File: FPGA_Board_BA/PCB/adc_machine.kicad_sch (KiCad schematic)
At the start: 6 parts, among them J201 PinHeader_03_male, U201 LTC2320-16_LVDS

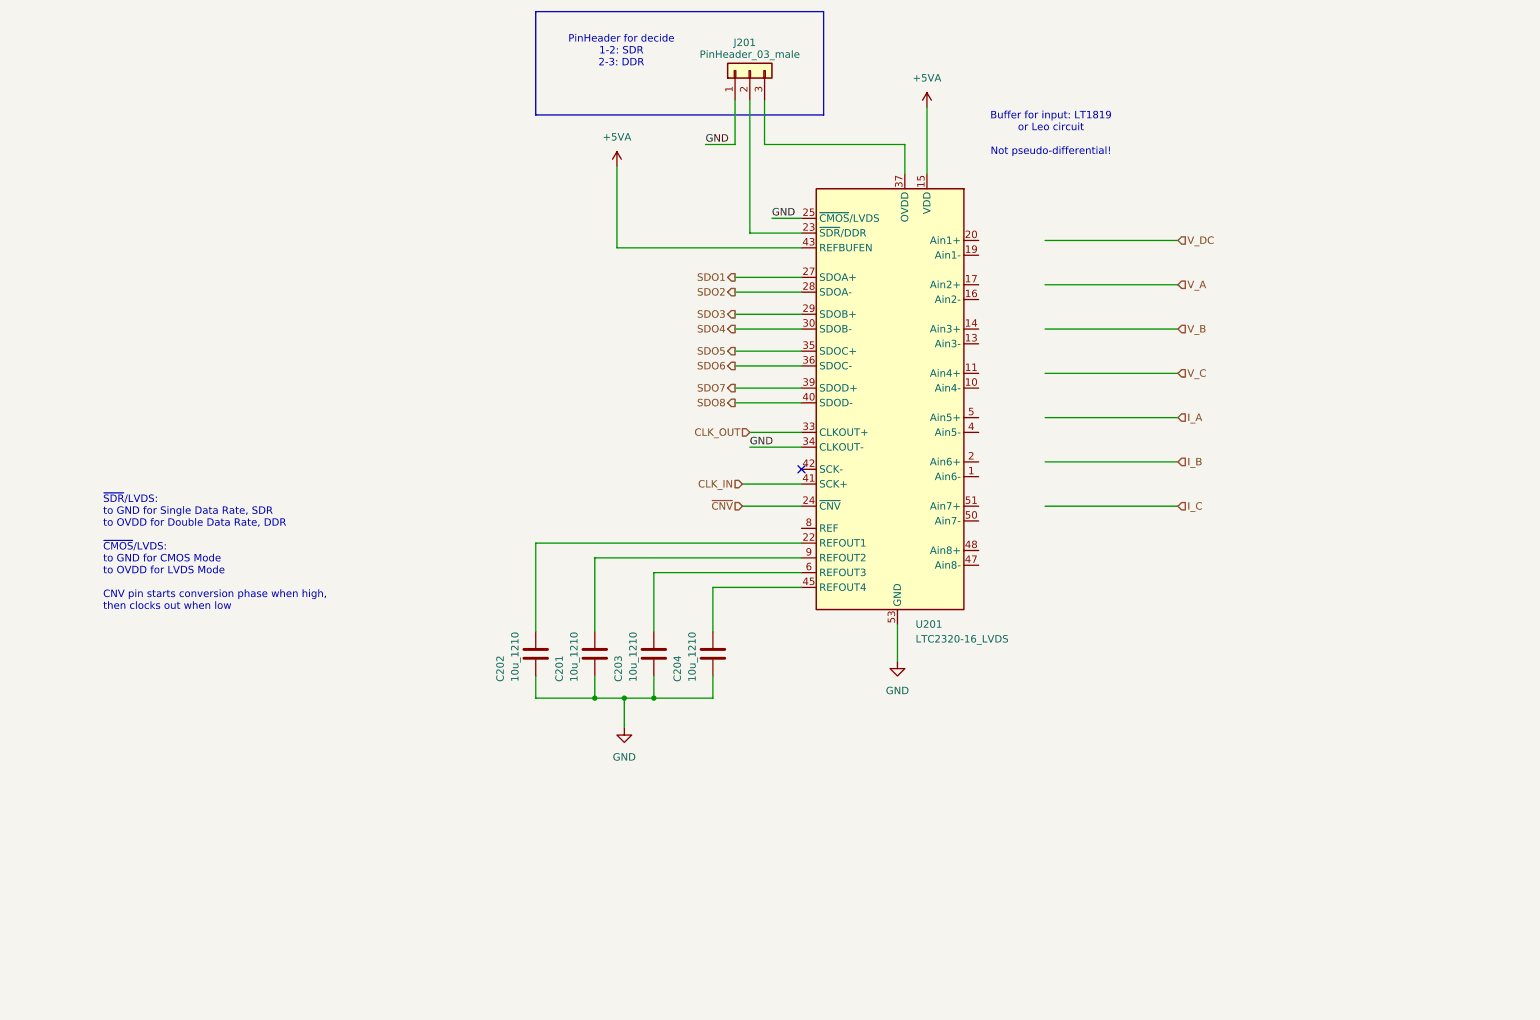
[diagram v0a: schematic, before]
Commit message: some schematic changes + Misc
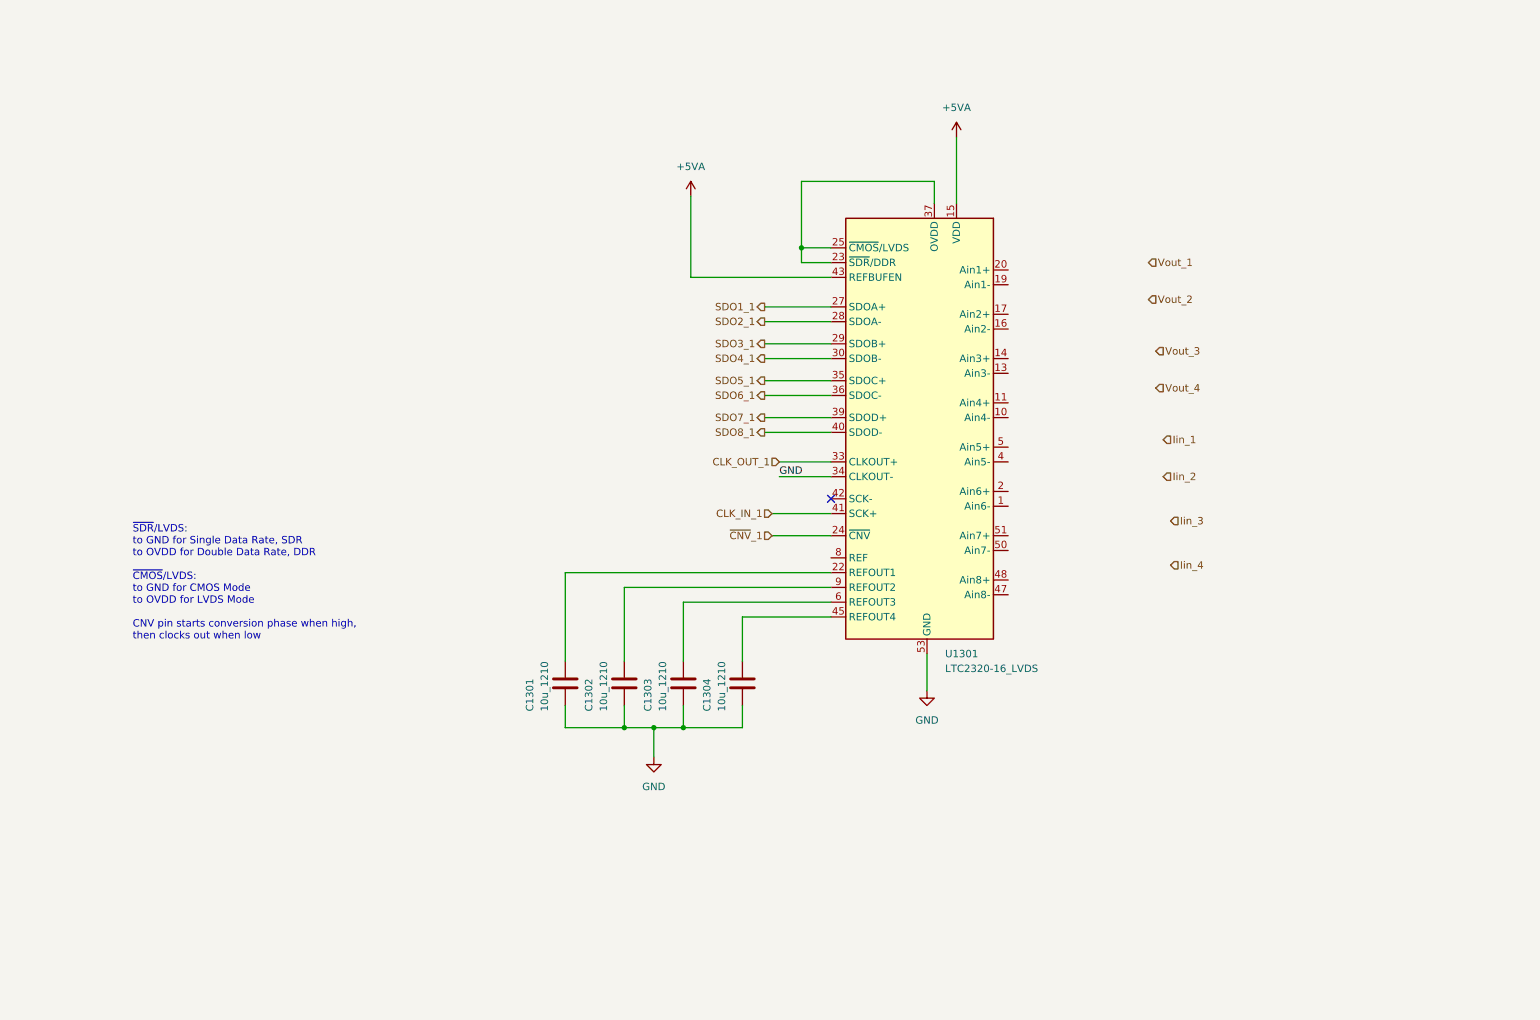
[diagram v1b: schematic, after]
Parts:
- removed C201, C202, C203, C204: 10u_1210, WLIB_Capacitor:C_1210, symbol WLIB_C:10u_1210
- removed J201: PinHeader_03_male, Connector_PinHeader_2.54mm:PinHeader_1x03_P2.54mm_Vertical, symbol WLIB_J:PinHeader_03_male
- removed U201: LTC2320-16_LVDS, MYLIB_chips:UKG_52_7mm_8mm, symbol MYLIB_U:LTC2320-16_LVDS
- added C1301, C1302, C1303, C1304: 10u_1210, WLIB_Capacitor:C_1210, symbol WLIB_C:10u_1210
- added U1301: LTC2320-16_LVDS, MYLIB_chips:UKG_52_7mm_8mm, symbol MYLIB_U:LTC2320-16_LVDS
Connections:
- net +5VA: now also U1301.15 (VDD), U1301.21 (VDD), U1301.43 (REFBUFEN), U1301.44 (VDD), U1301.52 (VDD)
- net GND: now also C1301.2, C1302.2, C1303.2, C1304.2, U1301.12 (GND), U1301.18 (GND), U1301.26 (GND), U1301.3 (GND), U1301.32 (GND), U1301.34 (CLKOUT-), U1301.38 (GND), U1301.46 (GND), U1301.49 (GND), U1301.53 (GND), U1301.7 (GND)
- net OVDD: now also U1301.23 (~{SDR}/DDR), U1301.25 (~{CMOS}/LVDS), U1301.31 (OVDD), U1301.37 (OVDD)
- new net: C1303.1, U1301.6 (REFOUT3)
- new net: C1301.1, U1301.22 (REFOUT1)
- new net: C1302.1, U1301.9 (REFOUT2)
- new net: C1304.1, U1301.45 (REFOUT4)
- new net CLK_IN_1: U1301.41 (SCK+)
- new net CLK_OUT_1: U1301.33 (CLKOUT+)
- new net SDO1_1: U1301.27 (SDOA+)
- new net SDO2_1: U1301.28 (SDOA-)
- new net SDO3_1: U1301.29 (SDOB+)
- new net SDO4_1: U1301.30 (SDOB-)
- new net SDO5_1: U1301.35 (SDOC+)
- new net SDO6_1: U1301.36 (SDOC-)
- new net SDO7_1: U1301.39 (SDOD+)
- new net SDO8_1: U1301.40 (SDOD-)
- new net ~{CNV}_1: U1301.24 (~{CNV})
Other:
- note removed: "Buffer for input: LT1819 or Leo circuit Not pseudo-differential!"
- note removed: "PinHeader for decide 1-2: SDR 2-3: DDR"

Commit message: lot of work
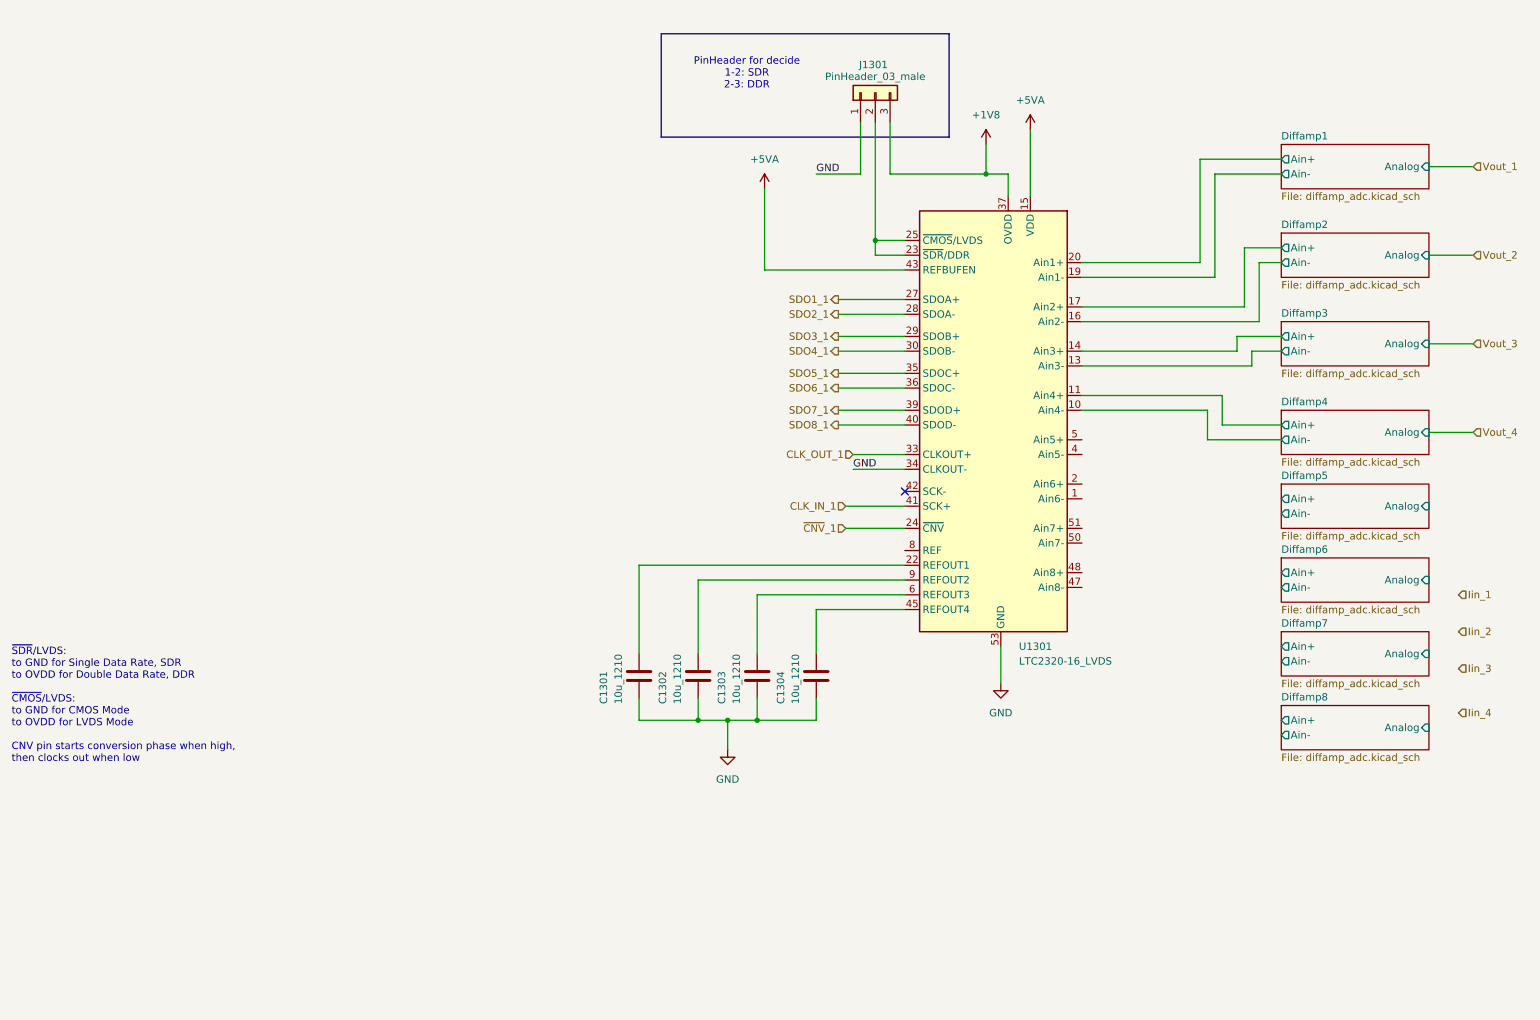
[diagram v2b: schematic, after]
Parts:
- added J1301: PinHeader_03_male, Connector_PinHeader_2.54mm:PinHeader_1x03_P2.54mm_Vertical, symbol WLIB_J:PinHeader_03_male
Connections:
- net GND: now also J1301.1 (Pin_1)
- net Diffamp4/Ain-: now reaches U1301.10 (Ain4-)
- net Diffamp4/Ain+: now reaches U1301.11 (Ain4+)
- net Diffamp3/Ain-: now reaches U1301.13 (Ain3-)
- net Diffamp3/Ain+: now reaches U1301.14 (Ain3+)
- net Diffamp2/Ain-: now reaches U1301.16 (Ain2-)
- net Diffamp2/Ain+: now reaches U1301.17 (Ain2+)
- net Diffamp1/Ain-: now reaches U1301.19 (Ain1-)
- net Diffamp1/Ain+: now reaches U1301.20 (Ain1+)
- net OVDD: no longer names the net of U1301.23 (~{SDR}/DDR), U1301.25 (~{CMOS}/LVDS)
- net OVDD: now also J1301.2 (Pin_2); no longer U1301.31 (OVDD), U1301.37 (OVDD)
- new net +1V8: J1301.3 (Pin_3), U1301.31 (OVDD), U1301.37 (OVDD)
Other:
- added sheet Diffamp1 (diffamp_adc.kicad_sch)
- added sheet Diffamp2 (diffamp_adc.kicad_sch)
- added sheet Diffamp3 (diffamp_adc.kicad_sch)
- added sheet Diffamp4 (diffamp_adc.kicad_sch)
- added sheet Diffamp5 (diffamp_adc.kicad_sch)
- added sheet Diffamp6 (diffamp_adc.kicad_sch)
- added sheet Diffamp7 (diffamp_adc.kicad_sch)
- added sheet Diffamp8 (diffamp_adc.kicad_sch)
- note added: "PinHeader for decide 1-2: SDR 2-3: DDR"
- moved on the sheet: C1301, C1302, C1303, C1304, U1301

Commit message: work
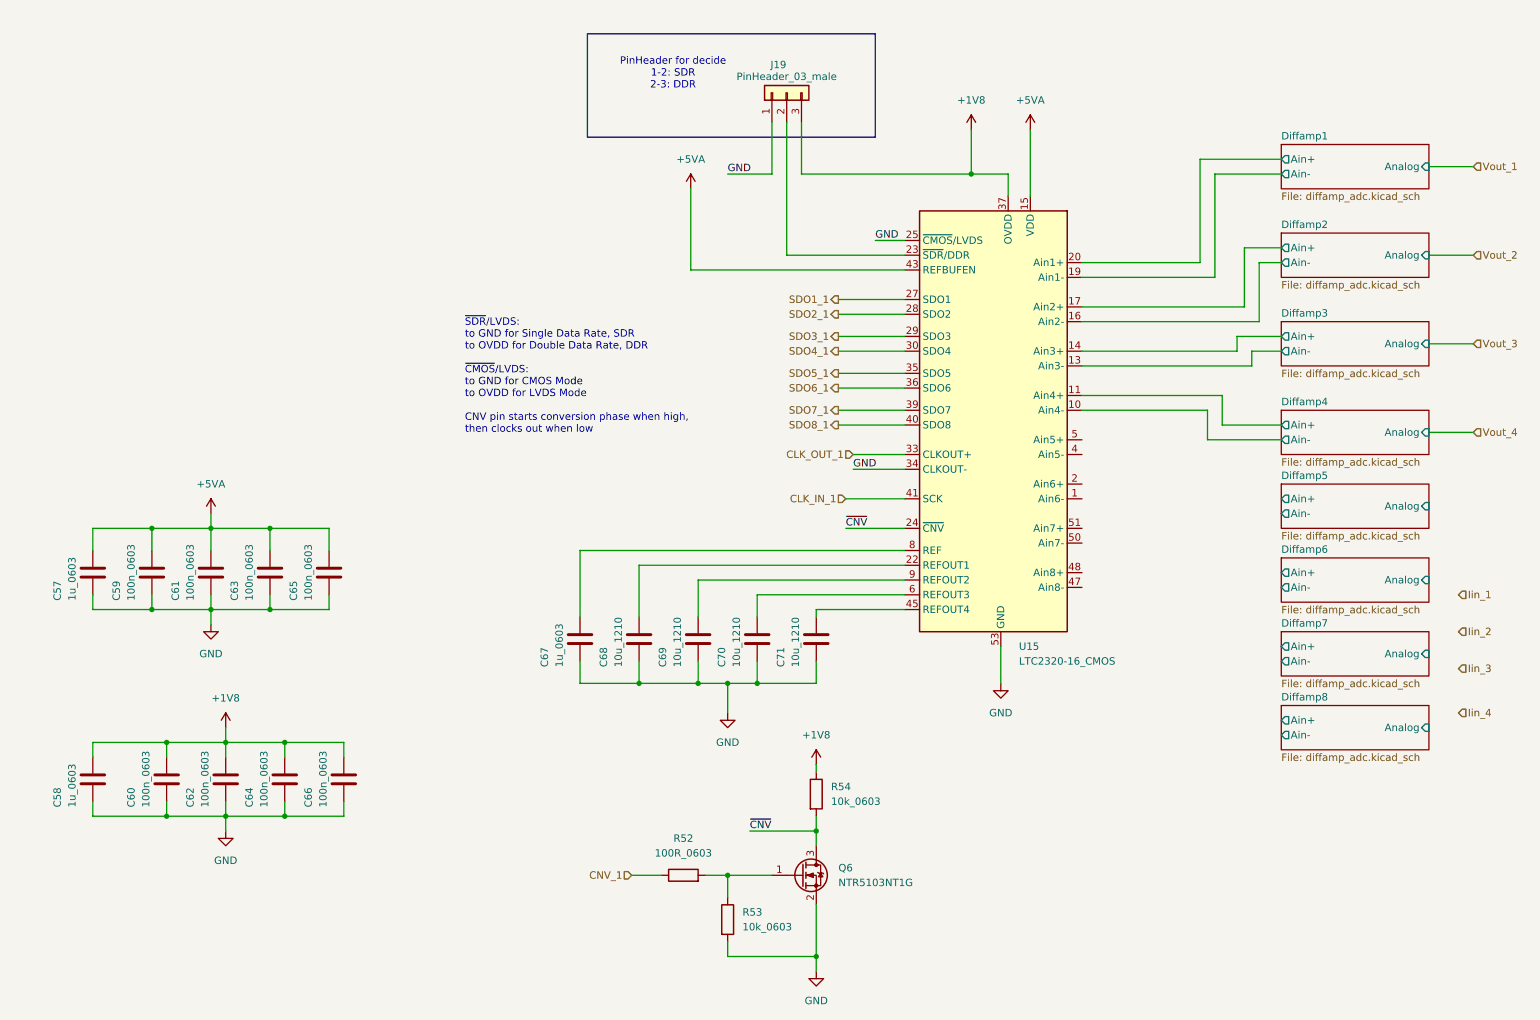
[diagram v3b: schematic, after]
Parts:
- removed U1301: LTC2320-16_LVDS, MYLIB_chips:UKG_52_7mm_8mm, symbol MYLIB_U:LTC2320-16_LVDS
- added C57, C58, C67: 1u_0603, WLIB_Capacitor:C_0603, symbol WLIB_C:1u_0603
- added C59, C60, C61, C62, C63, C64, C65, C66: 100n_0603, WLIB_Capacitor:C_0603, symbol WLIB_C:100n_0603
- added Q6: NTR5103NT1G, Package_TO_SOT_SMD:SOT-23_Handsoldering, symbol WLIB_Q:NTR5103NT1G
- added R52: 100R_0603, Resistor_SMD:R_0603_1608Metric, symbol WLIB_R:100R_0603
- added R53, R54: 10k_0603, Resistor_SMD:R_0603_1608Metric, symbol WLIB_R:10k_0603
- added U15: LTC2320-16_CMOS, MYLIB_chips:UKG_52_7mm_8mm, symbol MYLIB_U:LTC2320-16_CMOS
- renumbered C1301 to C68, C1302 to C69, C1303 to C70, C1304 to C71, J1301 to J19
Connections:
- net +1V8: now also C58.1, C60.1, C62.1, C64.1, C66.1, R54.1, U15.31 (OVDD), U15.37 (OVDD)
- net +5VA: now also C57.1, C59.1, C61.1, C63.1, C65.1, U15.15 (VDD), U15.21 (VDD), U15.43 (REFBUFEN), U15.44 (VDD), U15.52 (VDD)
- net CLK_IN_1: now also U15.41 (SCK)
- net CLK_OUT_1: now also U15.33 (CLKOUT+)
- net Diffamp1/Ain+: now also U15.20 (Ain1+)
- net Diffamp1/Ain-: now also U15.19 (Ain1-)
- net Diffamp2/Ain+: now also U15.17 (Ain2+)
- net Diffamp2/Ain-: now also U15.16 (Ain2-)
- net Diffamp3/Ain+: now also U15.14 (Ain3+)
- net Diffamp3/Ain-: now also U15.13 (Ain3-)
- net Diffamp4/Ain+: now also U15.11 (Ain4+)
- net Diffamp4/Ain-: now also U15.10 (Ain4-)
- net GND: now also C57.2, C58.2, C59.2, C60.2, C61.2, C62.2, C63.2, C64.2, C65.2, C66.2, C67.2, Q6.2 (S), R53.2, U15.12 (GND), U15.18 (GND), U15.25 (~{CMOS}/LVDS), U15.26 (GND), U15.3 (GND), U15.32 (GND), U15.34 (CLKOUT-), U15.38 (GND), U15.46 (GND), U15.49 (GND), U15.53 (GND), U15.7 (GND)
- net SDO1_1: now also U15.27 (SDO1)
- net SDO2_1: now also U15.28 (SDO2)
- net SDO3_1: now also U15.29 (SDO3)
- net SDO4_1: now also U15.30 (SDO4)
- net SDO5_1: now also U15.35 (SDO5)
- net SDO6_1: now also U15.36 (SDO6)
- net SDO7_1: now also U15.39 (SDO7)
- net SDO8_1: now also U15.40 (SDO8)
- net at C70.1: now also U15.6 (REFOUT3)
- net at C68.1: now also U15.22 (REFOUT1)
- net at C69.1: now also U15.9 (REFOUT2)
- net at J19.2 (Pin_2): now also U15.23 (~{SDR}/DDR)
- net at C71.1: now also U15.45 (REFOUT4)
- new net: Q6.1 (G), R52.2, R53.1
- new net: C67.1, U15.8 (REF)
- new net CNV_1: R52.1
- new net ~{CNV}: Q6.3 (D), R54.2, U15.24 (~{CNV})
- no-connect marks 1 -> 0
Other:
- moved on the sheet: C68, C69, C70, C71, J19
